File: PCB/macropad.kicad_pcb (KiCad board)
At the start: 2 copper layers, 63 x 81.4 mm, 11 parts, among them SW1 SW_Push, SW2 SW_Push, SW3 SW_Push, SW4 SW_Push, SW5 SW_Push, SW6 SW_Push, SW7 SW_Push, SW8 SW_Push, SW9 SW_Push, U1 XIAO-RP2040-DIP

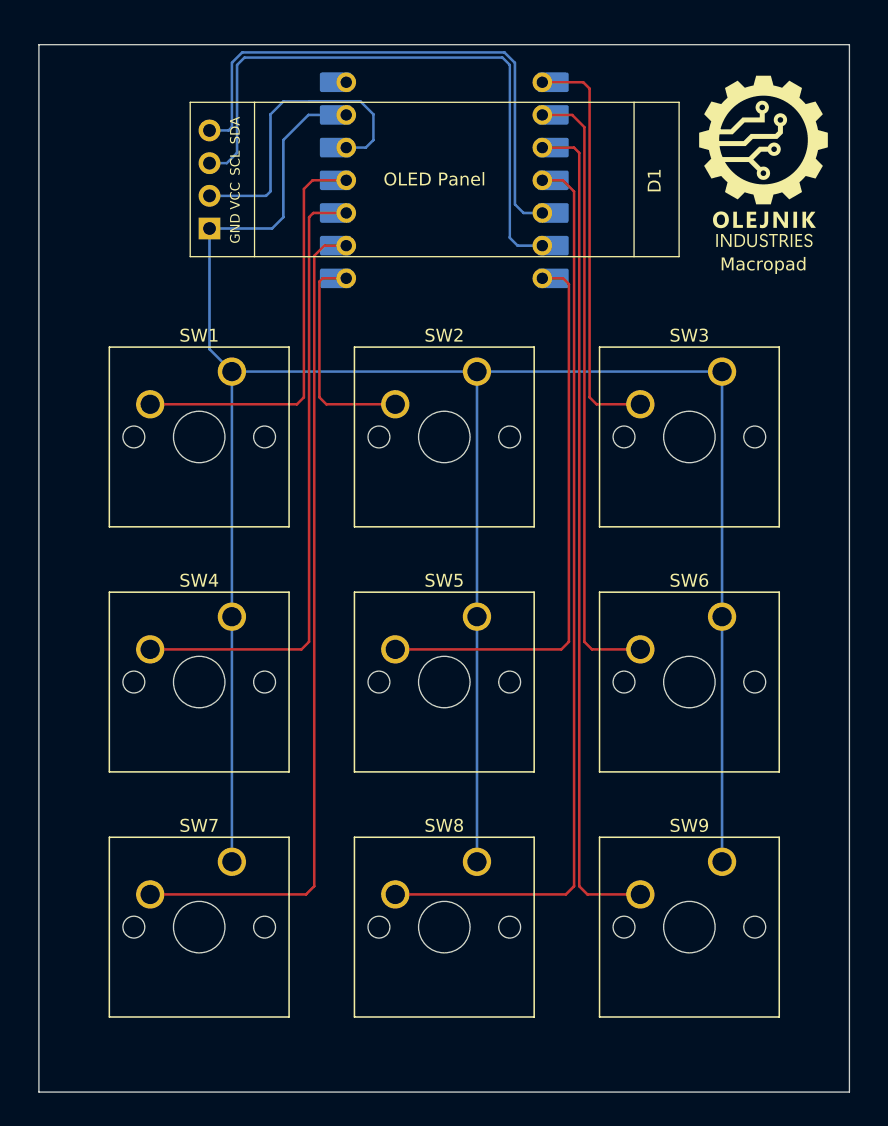
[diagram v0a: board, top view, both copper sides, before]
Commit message: PCB v.2
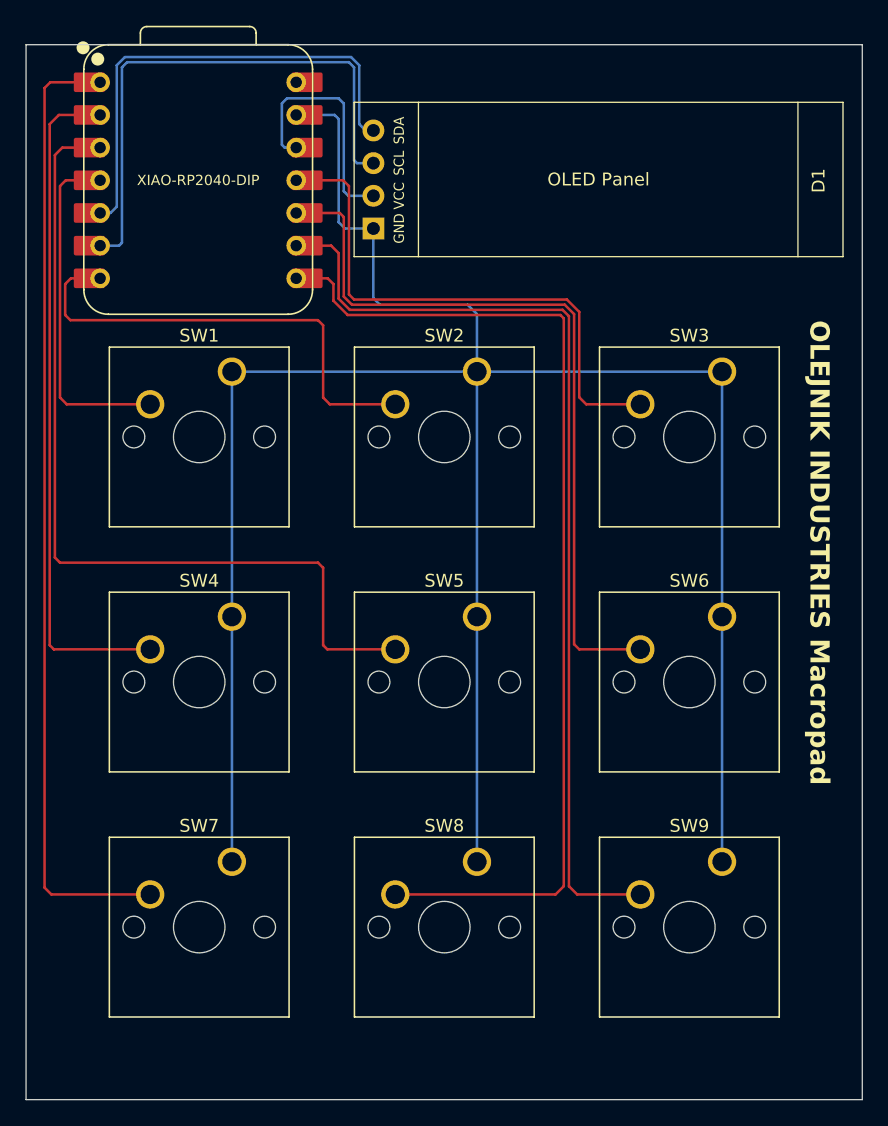
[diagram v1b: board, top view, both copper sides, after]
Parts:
- U1: moved to F.Cu
- moved U1 19.1 mm to (107.4, 70.1), turned to 0 degrees
- moved D1 12.7 mm to (157.5, 76.1)
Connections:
- SW1 pad 2: Net-(U1-GPIO3/MOSI) -> Net-(U1-GPIO29/ADC3/A3)
- SW2 pad 2: Net-(U1-GPIO1/RX) -> Net-(U1-GPIO0/TX)
- SW3 pad 2: Net-(U1-GPIO26/ADC0/A0) -> Net-(U1-GPIO3/MOSI)
- SW4 pad 2: Net-(U1-GPIO4/MISO) -> Net-(U1-GPIO27/ADC1/A1)
- SW5 pad 2: Net-(U1-GPIO0/TX) -> Net-(U1-GPIO28/ADC2/A2)
- SW6 pad 2: Net-(U1-GPIO27/ADC1/A1) -> Net-(U1-GPIO4/MISO)
- SW7 pad 2: Net-(U1-GPIO2/SCK) -> Net-(U1-GPIO26/ADC0/A0)
- SW8 pad 2: Net-(U1-GPIO29/ADC3/A3) -> Net-(U1-GPIO1/RX)
- SW9 pad 2: Net-(U1-GPIO28/ADC2/A2) -> Net-(U1-GPIO2/SCK)
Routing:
- net Net-(U1-GPIO1/RX): track 17.3 -> 80.3 mm
- net Net-(U1-GPIO29/ADC3/A3): track 71.0 -> 26.1 mm
- net Net-(U1-GPIO26/ADC0/A0): track 32.0 -> 75.1 mm
- net Net-(U1-GPIO2/SCK): track 64.8 -> 75.7 mm
- net Net-(U1-GPIO4/MISO): track 48.6 -> 59.5 mm
- net Net-(U1-GPIO3/MOSI): track 31.9 -> 41.9 mm
- net Net-(U1-GPIO0/TX): track 43.8 -> 36.3 mm
- net /VCC: track 24.1 -> 18.8 mm
- net /SDA: track 42.9 -> 37.7 mm
- net /SCL: track 47.2 -> 42.6 mm
- net Net-(U1-GPIO27/ADC1/A1): track 48.3 -> 52.7 mm
- net GND: track 182.0 -> 185.2 mm
- net Net-(U1-GPIO28/ADC2/A2): track 65.1 -> 68.0 mm
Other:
- board size 63 x 81.4 mm -> 65 x 82 mm
- board text added: "OLEJNIK INDUSTRIES Macropad"
